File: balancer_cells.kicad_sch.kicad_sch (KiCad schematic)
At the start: 22 parts, among them U3 BQ76952PFBR

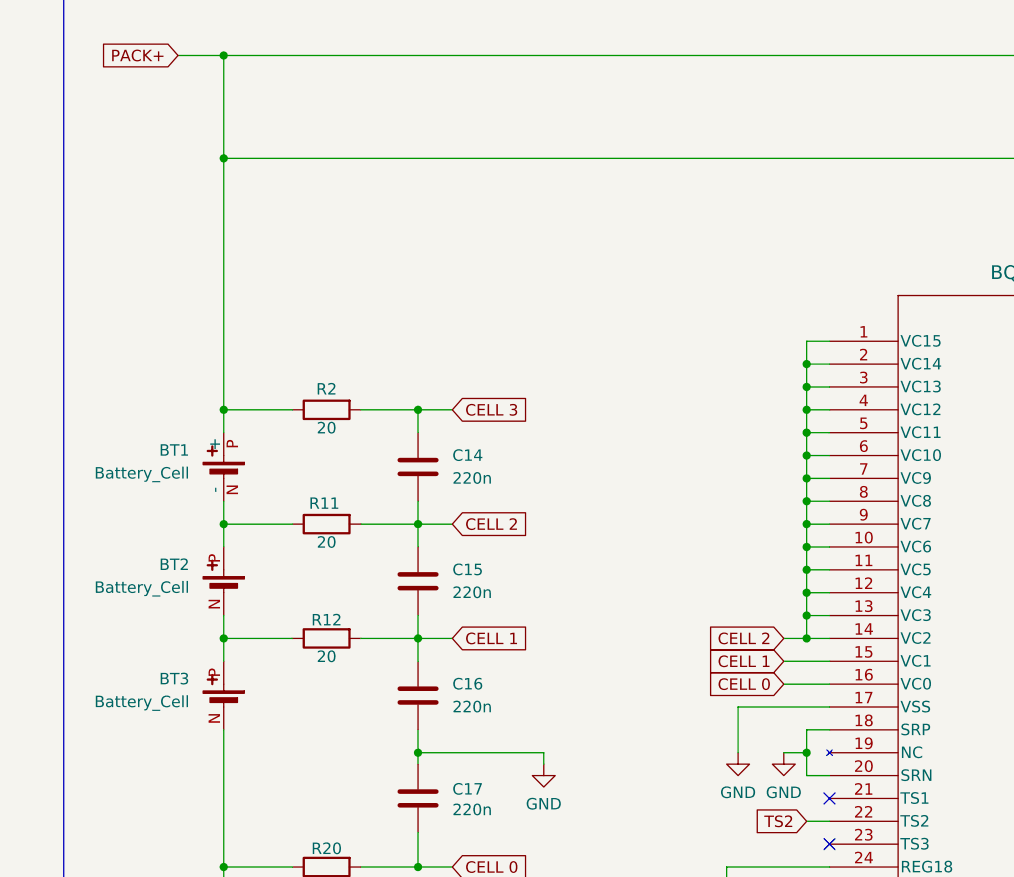
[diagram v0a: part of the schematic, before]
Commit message: added todos
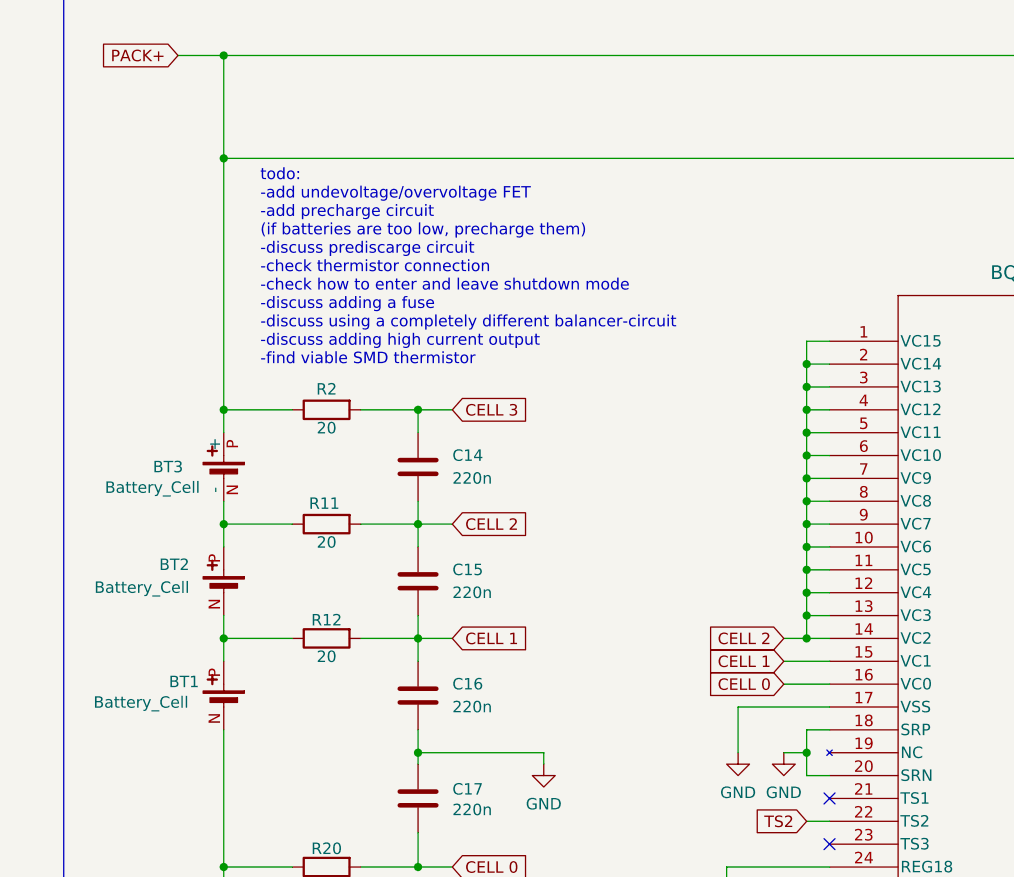
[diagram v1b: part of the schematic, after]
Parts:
- renumbered BT3 to BT1, BT1 to BT3
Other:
- note added: "todo: -add undevoltage/overvoltage FET -add precharge circuit (if batteries are too low, precharge them) -discuss prediscarge circuit -check thermistor connection -check how to enter and leave shutdown mode -discuss adding a fuse -discuss using a completely different balancer-circuit -discuss adding high current output -find viable SMD thermistor"
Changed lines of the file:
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@@
+		)
+	)
+	(text "todo:\n-add undevoltage/overvoltage FET\n-add precharge circuit\n(if batteries are too low, precharge them)\n-discuss prediscarge circuit\n-check thermistor connection\n-check how to enter and leave shutdown mode\n-discuss adding a fuse\n-discuss using a completely different balancer-circuit\n-discuss adding high current output\n-find viable SMD thermistor"
+		(exclude_from_sim no)
+		(at 54.864 61.722 0)
+		(effects
+			(font
+				(size 1.27 1.27)
+			)
+			(justify left)
 		)
 	)
@@
 		(on_board yes)
 		(dnp no)
-		(fields_autoplaced yes)
-		(property "Reference" "BT3"
-			(at 46.99 107.3784 0)
-			(effects
-				(font
-					(size 1.27 1.27)
-				)
-				(justify left)
+		(property "Reference" "BT1"
+			(at 44.704 107.696 0)
+			(effects
+				(font
+					(size 1.27 1.27)
+				)
+				(justify right)
 			)
 		)
 		(property "Value" "Battery_Cell"
-			(at 46.99 109.9184 0)
-			(effects
-				(font
-					(size 1.27 1.27)
-				)
-				(justify left)
+			(at 36.322 109.982 0)
+			(effects
+				(font
+					(size 1.27 1.27)
+				)
+				(justify right)
 			)
 		)
@@
 			(project "rapid_power_module"
 				(path "/afc8cbd3-9ea8-40a2-afae-ed6bd0fe7e6e/bfae272a-4bf5-4960-b276-b4c1a7fb3062"
-					(reference "BT3")
+					(reference "BT1")
 					(unit 1)
 				)
@@
 		(on_board yes)
 		(dnp no)
-		(fields_autoplaced yes)
-		(property "Reference" "BT1"
-			(at 46.99 81.9784 0)
-			(effects
-				(font
-					(size 1.27 1.27)
-				)
-				(justify left)
+		(property "Reference" "BT3"
+			(at 42.926 83.82 0)
+			(effects
+				(font
+					(size 1.27 1.27)
+				)
+				(justify right)
 			)
 		)
 		(property "Value" "Battery_Cell"
-			(at 46.99 84.5184 0)
-			(effects
-				(font
-					(size 1.27 1.27)
-				)
-				(justify left)
+			(at 37.592 86.106 0)
+			(effects
+				(font
+					(size 1.27 1.27)
+				)
+				(justify right)
 			)
 		)
@@
 			(project "rapid_power_module"
 				(path "/afc8cbd3-9ea8-40a2-afae-ed6bd0fe7e6e/bfae272a-4bf5-4960-b276-b4c1a7fb3062"
-					(reference "BT1")
+					(reference "BT3")
 					(unit 1)
 				)
